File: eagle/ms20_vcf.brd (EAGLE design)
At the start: 100 x 80 mm, 41 parts, among them IC1 LM13700N, IC2 TL082P, IC3 TL082P, Q1 BC559C, Q2 BC559C

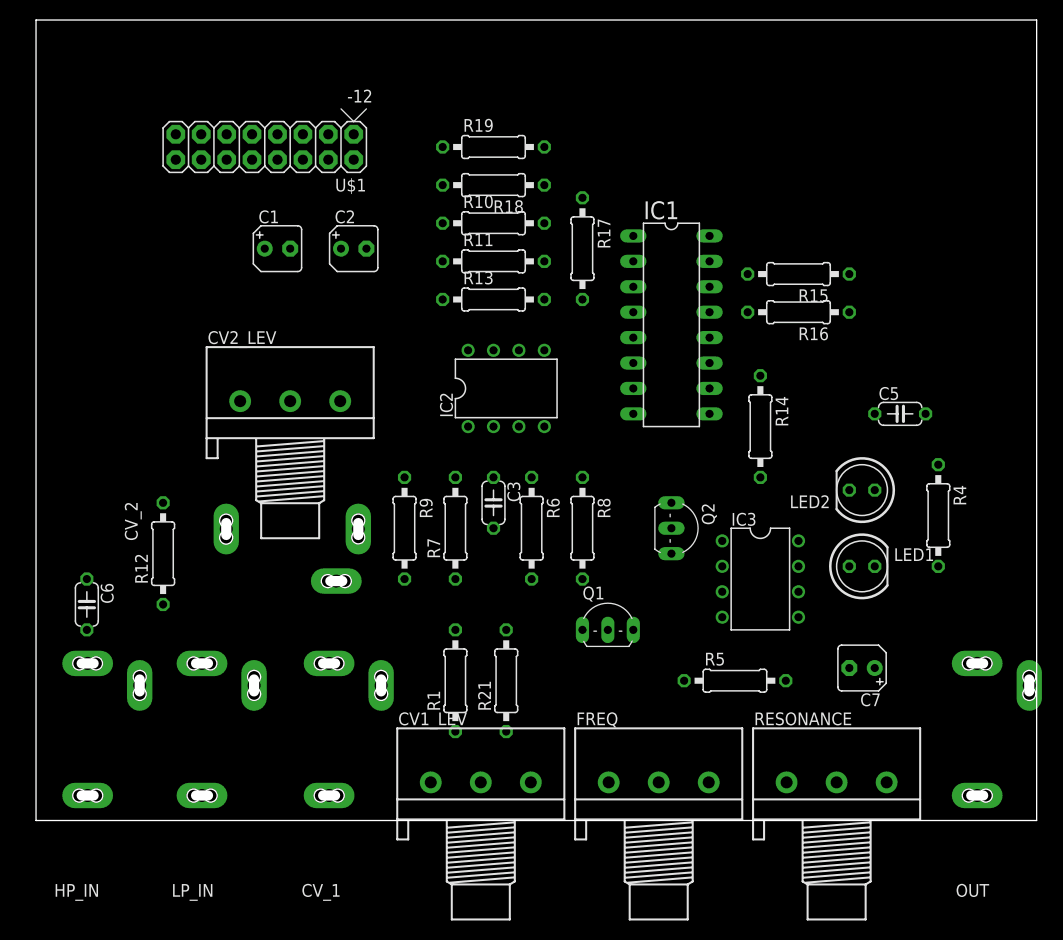
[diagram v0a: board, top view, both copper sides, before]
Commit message: routed
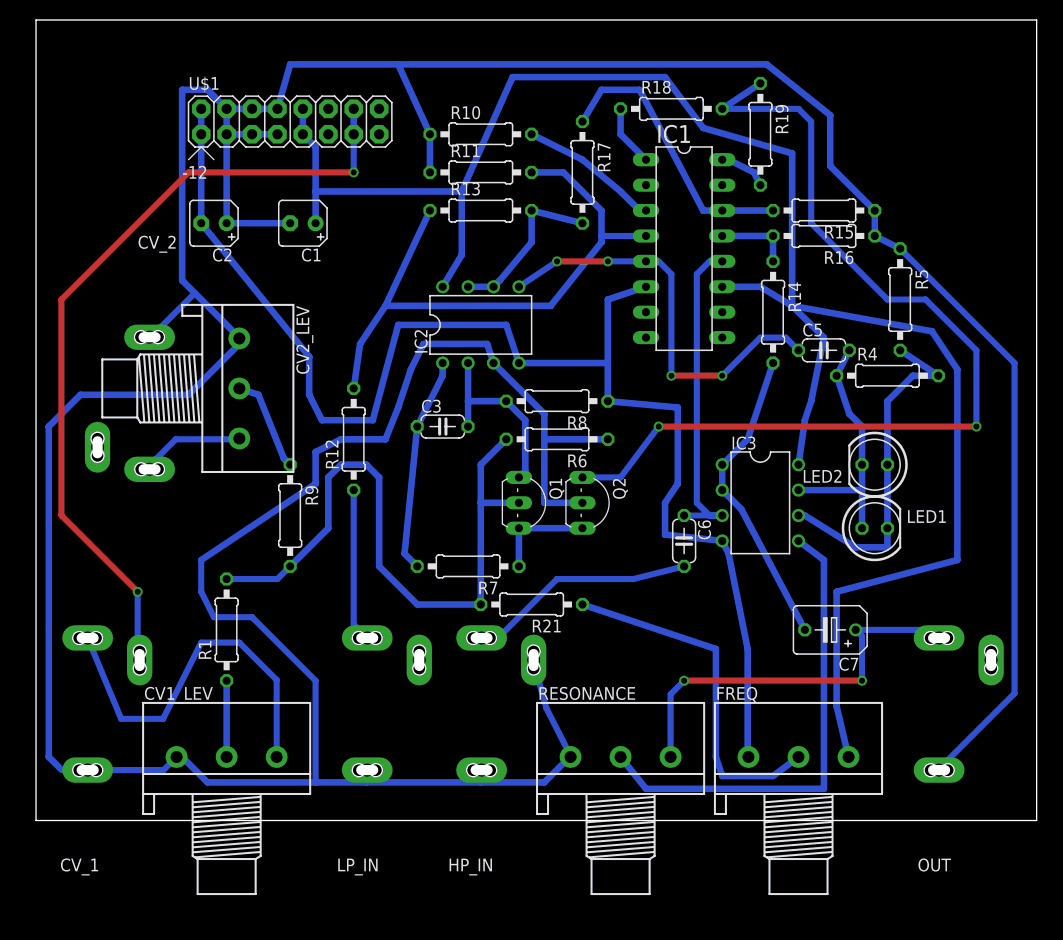
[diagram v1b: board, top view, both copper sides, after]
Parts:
- C7: device rcl:B45181A -> rcl:B45181B
- moved C6 60.0 mm to (64.8, 27.9)
- moved R5 41.5 mm to (86.4, 52.1), turned to 270 degrees
- moved HP_IN 39.5 mm to (49.5, 2.54)
- moved CV_2 28.5 mm to (6.35, 50.8), turned to 0 degrees
- moved R19 26.7 mm to (72.4, 68.6), turned to 270 degrees
- moved CV1_LEV 25.5 mm to (19.1, 6.35)
- moved CV_1 24.3 mm to (10.2, 2.54)
- moved R1 23.4 mm to (19.1, 19.1)
- moved R12 22.2 mm to (31.8, 38.1)
- moved RESONANCE 21.7 mm to (58.4, 6.35)
- moved R18 19.3 mm to (63.5, 71.1), turned to 0 degrees
- moved LP_IN 16.7 mm to (38.1, 2.54)
- moved R4 14.9 mm to (85.1, 44.5), turned to 0 degrees
- moved FREQ 14.2 mm to (76.2, 6.35)
- moved C2 14.2 mm to (17.8, 59.7), turned to 180 degrees
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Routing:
- net GND: track 0.00 -> 436.4 mm
- net +12V: track 0.00 -> 187.1 mm
- net -12V: track 0.00 -> 135.9 mm
- net N$16: track 0.00 -> 95.5 mm, vias 0 -> 2
- net N$27: track 0.00 -> 80.1 mm, vias 0 -> 2
- net N$21: track 0.00 -> 65.5 mm
- net N$14: track 0.00 -> 60.4 mm
- net N$6: track 0.00 -> 47.9 mm
- net N$9: track 0.00 -> 41.5 mm, vias 0 -> 4
- net N$12: track 0.00 -> 40.0 mm, vias 0 -> 2
- net N$24: track 0.00 -> 38.2 mm
- net N$1: track 0.00 -> 35.1 mm
- net N$22: track 0.00 -> 35.1 mm
- net N$10: track 0.00 -> 32.8 mm
- net N$11: track 0.00 -> 30.5 mm
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
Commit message: rerouted and milling
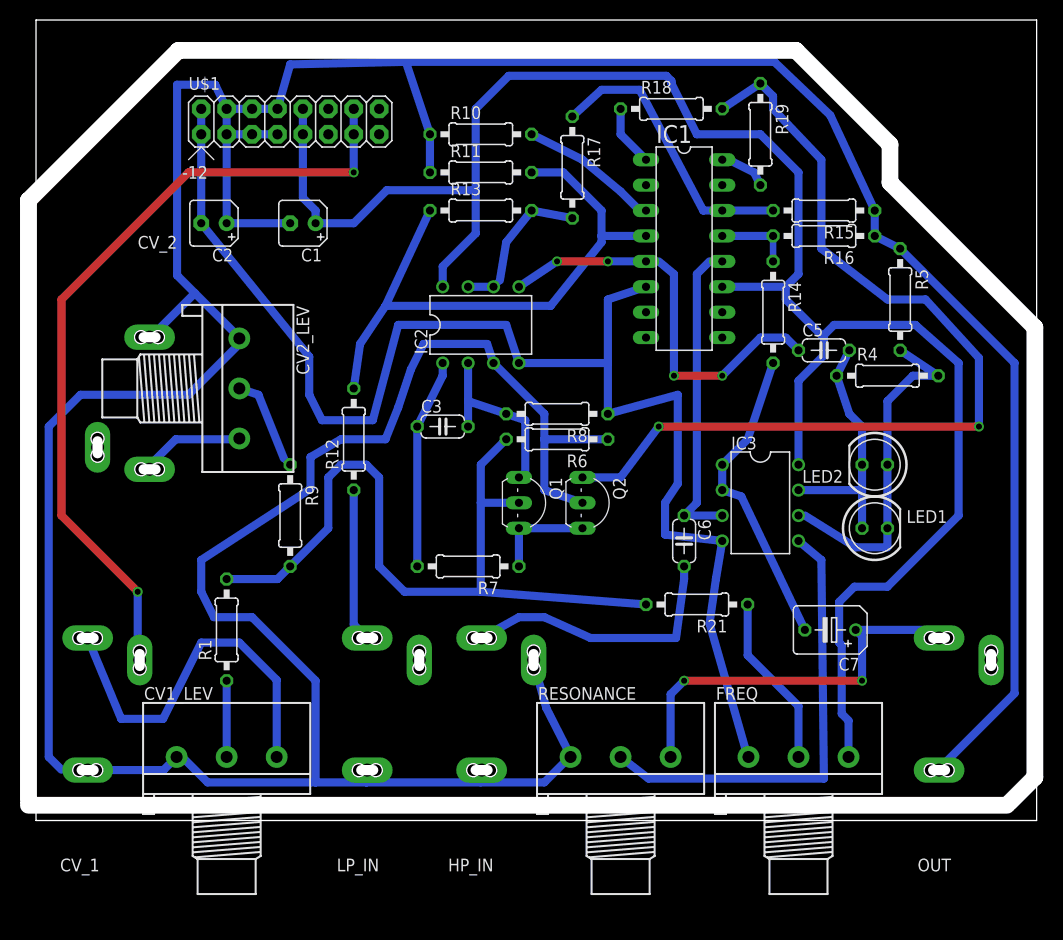
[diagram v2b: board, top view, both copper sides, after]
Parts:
- moved R21 16.5 mm to (66.0, 21.6)
- moved R8 1.27 mm to (52.1, 40.6)
- moved R17 1.14 mm to (53.6, 65.3)
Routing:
- net N$22: track 35.1 -> 17.3 mm
- net N$21: track 65.5 -> 80.2 mm
- net N$26: track 22.8 -> 27.6 mm
- net -12V: track 135.9 -> 139.0 mm
- net N$16: track 95.5 -> 92.6 mm
- net N$6: track 47.9 -> 45.9 mm
- net N$19: track 16.8 -> 15.5 mm
- net N$10: track 32.8 -> 31.5 mm
- net +12V: track 187.1 -> 188.2 mm
- net N$4: track 21.5 -> 20.9 mm
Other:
- board size 100 x 80 mm -> 100.8 x 80 mm
